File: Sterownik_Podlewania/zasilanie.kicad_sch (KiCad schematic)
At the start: 12 parts, among them J14 Screw_Terminal_01x02, J15 Barrel_Jack_MountingPin, J16 Screw_Terminal_01x02, SW8 SW_Push_DPDT, U3 L7805, U4 LM1117DT-3.3

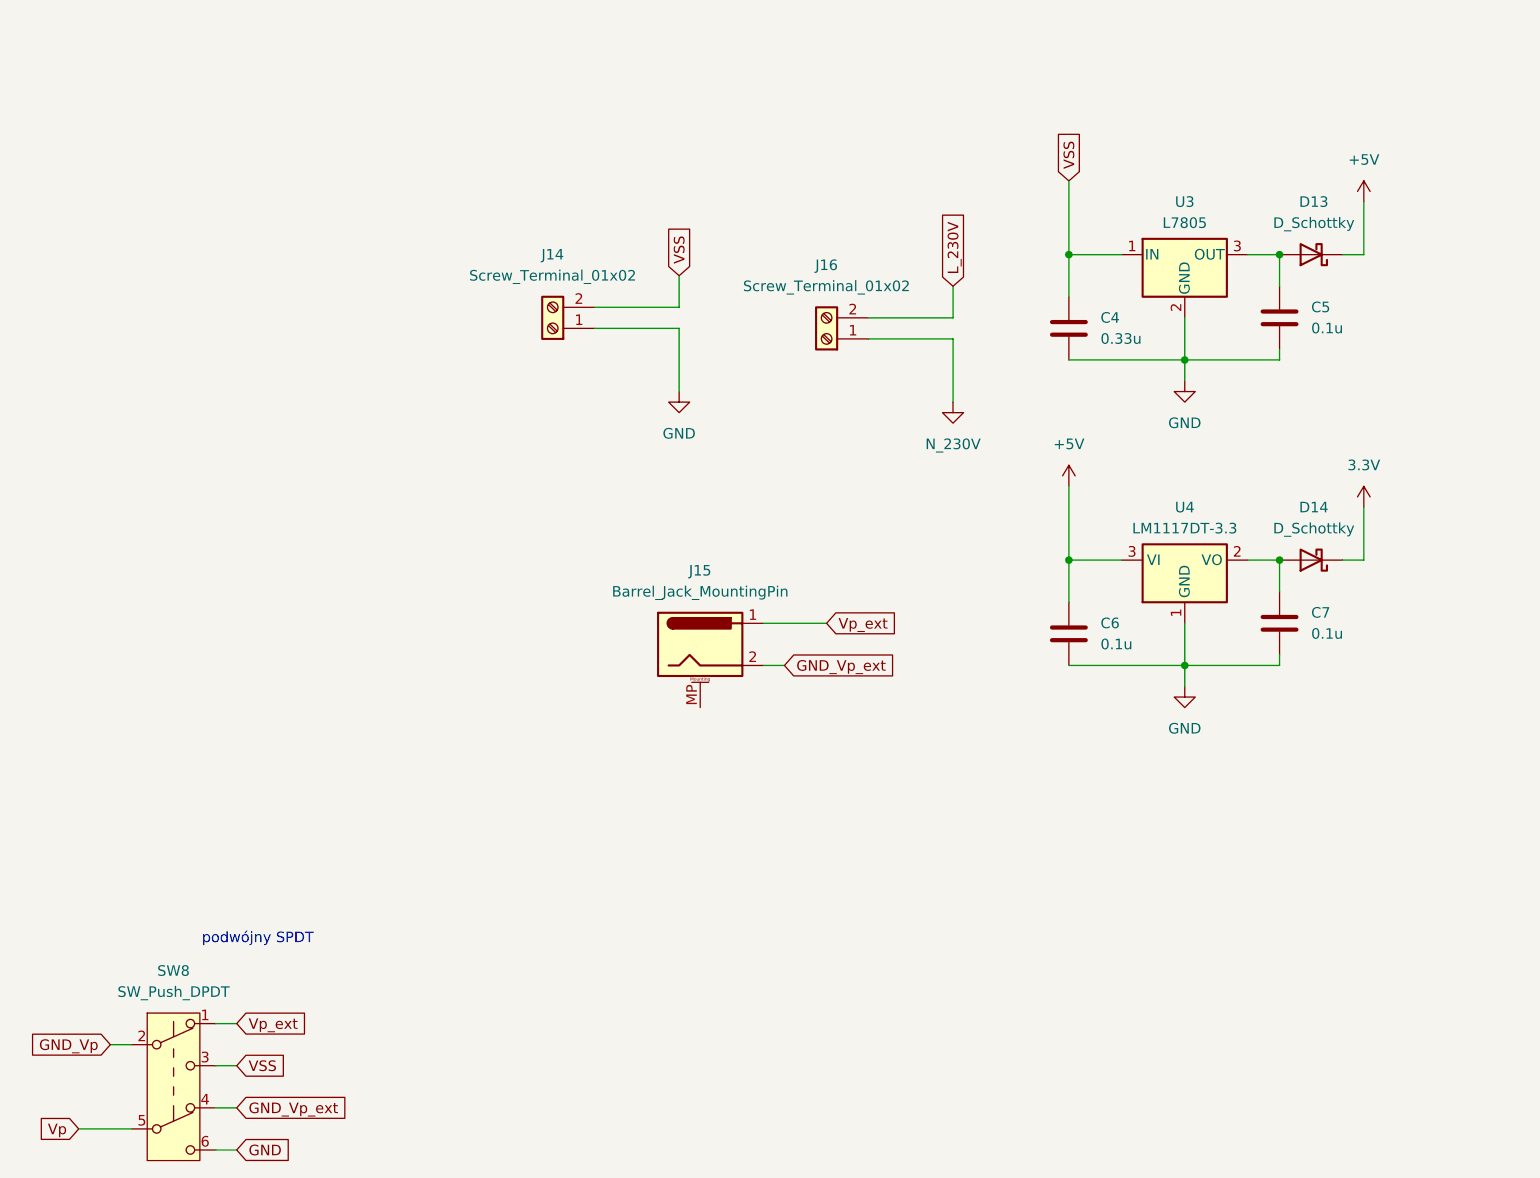
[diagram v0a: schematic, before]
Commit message: Poprawki estetyczne schematu
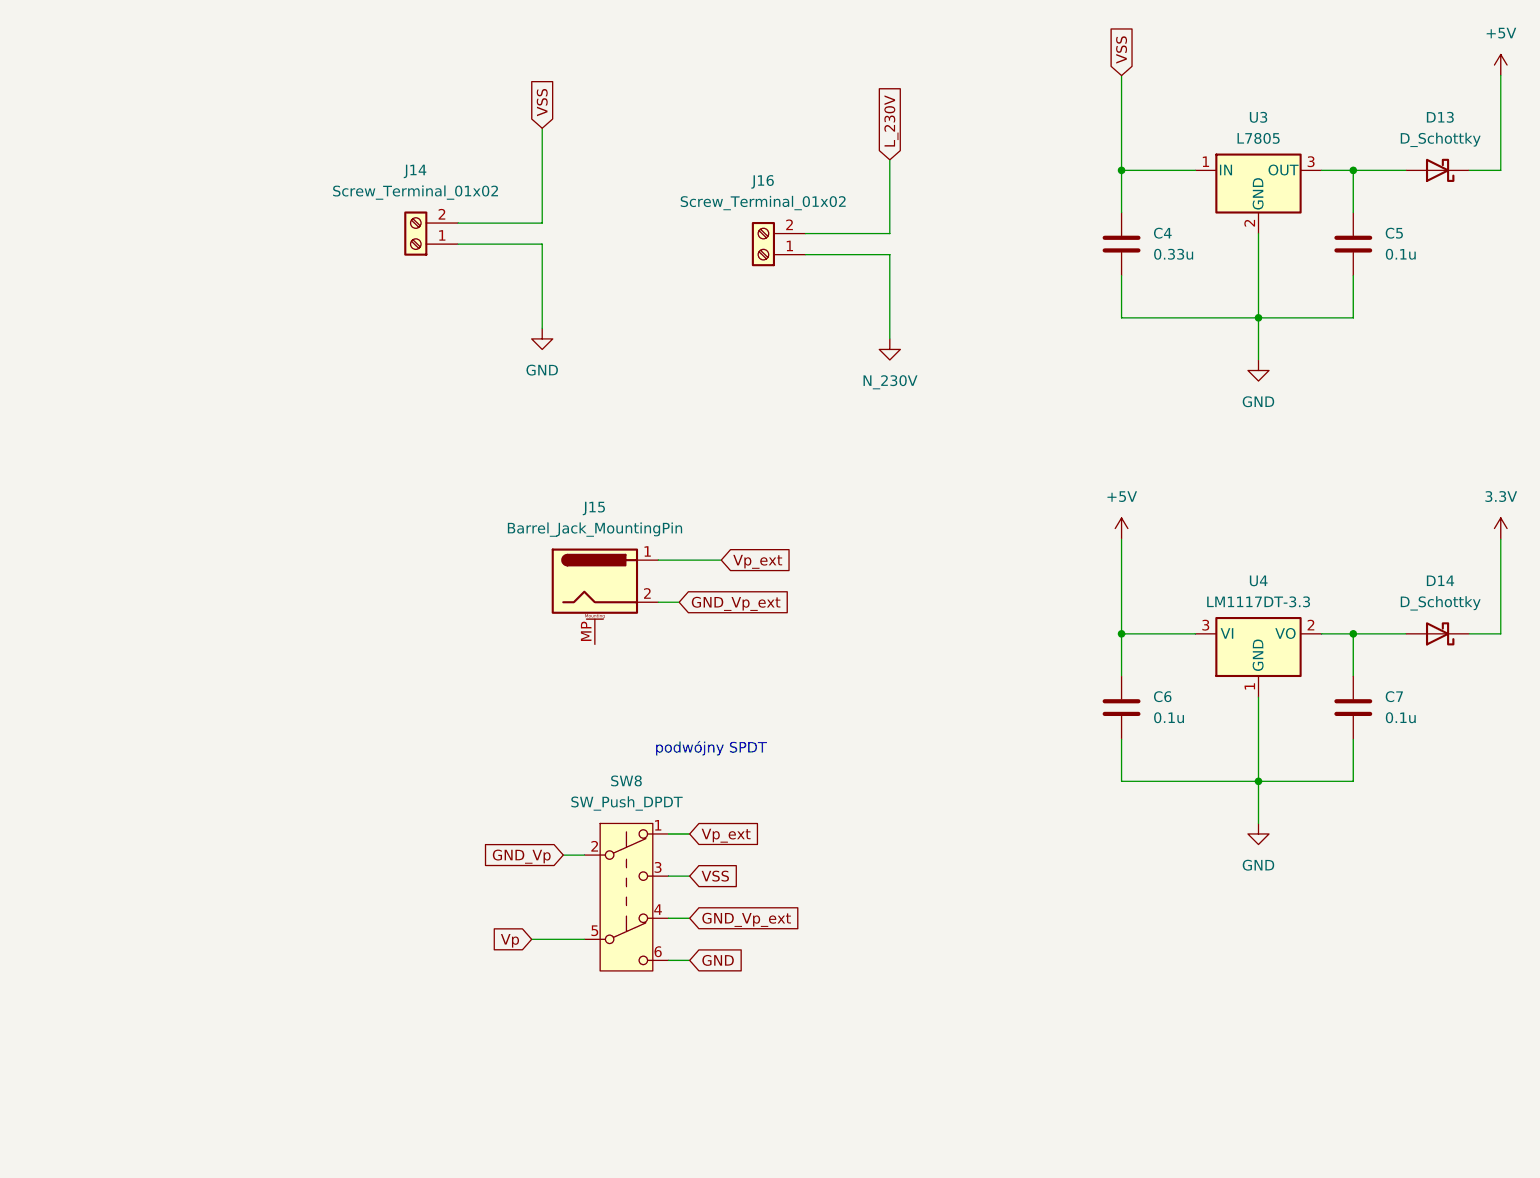
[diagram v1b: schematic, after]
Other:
- moved on the sheet: C4, C5, C6, C7, D13, D14, J14, J15, J16, SW8, U3, U4
